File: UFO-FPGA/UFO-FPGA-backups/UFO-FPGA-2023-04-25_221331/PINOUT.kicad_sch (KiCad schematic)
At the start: 4 parts, among them J2 Power, J3 Digital, J4 Digital/PWM, J5 Digital

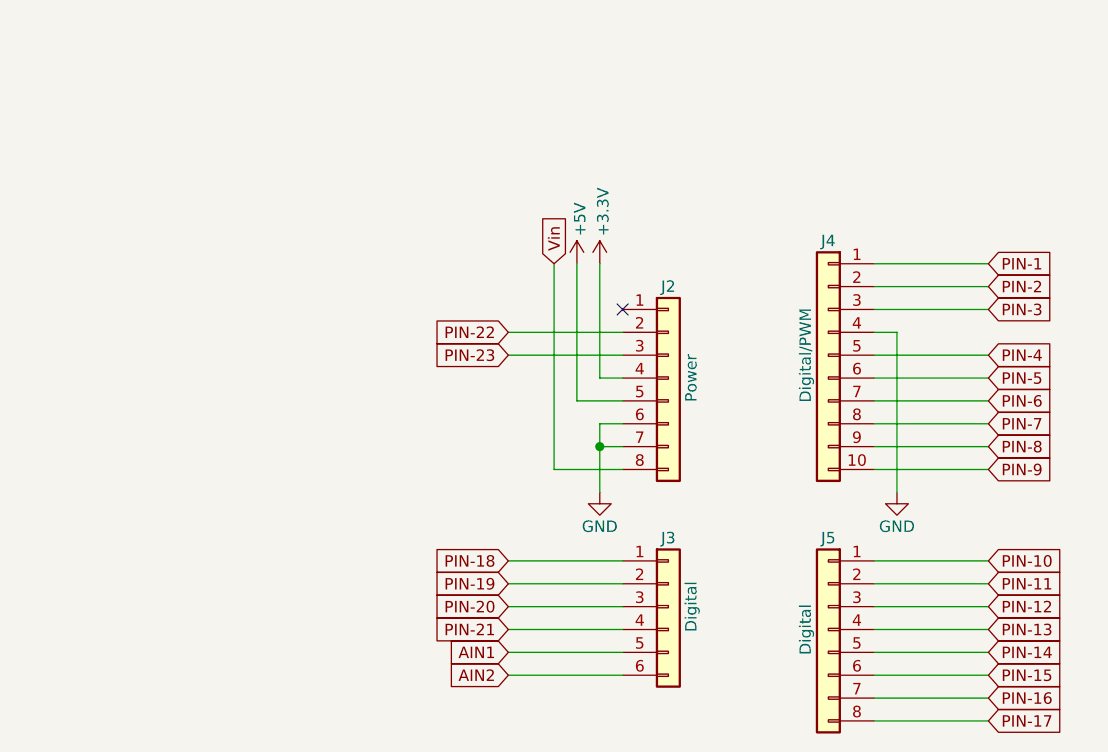
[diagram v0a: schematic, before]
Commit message: IO and power
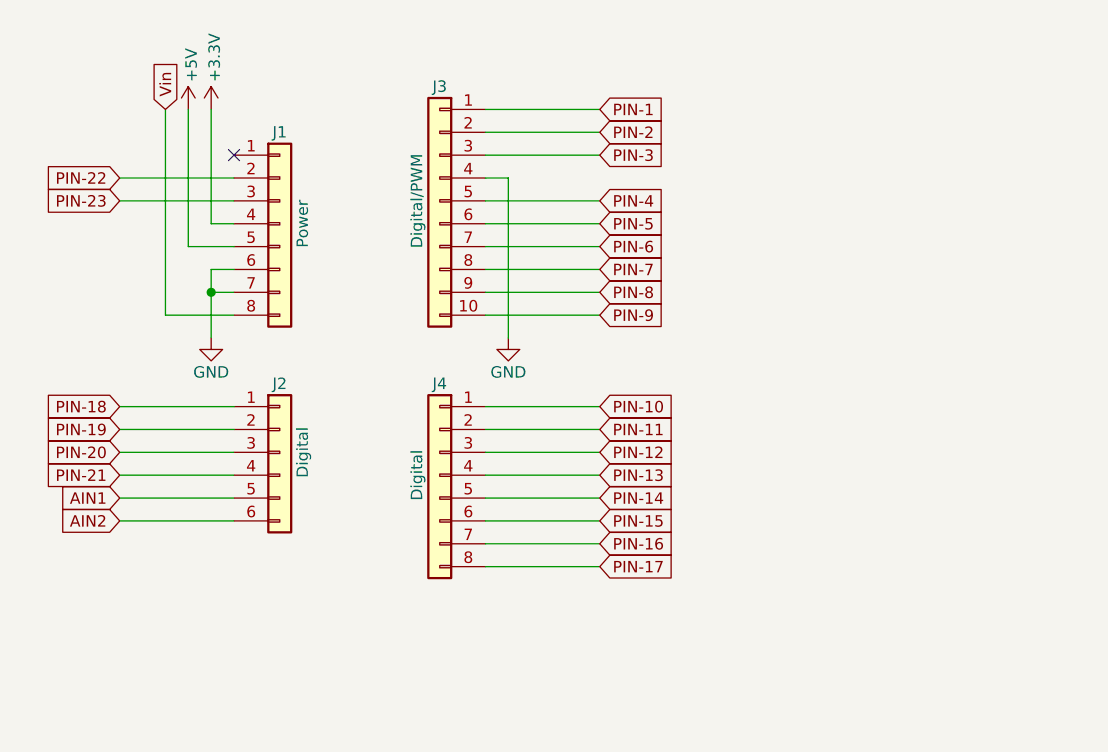
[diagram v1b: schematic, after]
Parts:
- removed J2: Power, Connector_PinSocket_2.54mm:PinSocket_1x08_P2.54mm_Vertical, symbol Connector_Generic:Conn_01x08
- removed J3: Digital, Connector_PinSocket_2.54mm:PinSocket_1x06_P2.54mm_Vertical, symbol Connector_Generic:Conn_01x06
- removed J4: Digital/PWM, Connector_PinSocket_2.54mm:PinSocket_1x10_P2.54mm_Vertical, symbol Connector_Generic:Conn_01x10
- removed J5: Digital, Connector_PinSocket_2.54mm:PinSocket_1x08_P2.54mm_Vertical, symbol Connector_Generic:Conn_01x08
- added J1: Power, Connector_PinSocket_2.54mm:PinSocket_1x08_P2.54mm_Vertical, symbol Connector_Generic:Conn_01x08
- added J2: Digital, Connector_PinSocket_2.54mm:PinSocket_1x06_P2.54mm_Vertical, symbol Connector_Generic:Conn_01x06
- added J3: Digital/PWM, Connector_PinSocket_2.54mm:PinSocket_1x10_P2.54mm_Vertical, symbol Connector_Generic:Conn_01x10
- added J4: Digital, Connector_PinSocket_2.54mm:PinSocket_1x08_P2.54mm_Vertical, symbol Connector_Generic:Conn_01x08
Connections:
- net +3V3: now also J1.4 (Pin_4)
- net +5V: now also J1.5 (Pin_5)
- net AIN1: now also J2.5 (Pin_5)
- net AIN2: now also J2.6 (Pin_6)
- net GND: now also J1.6 (Pin_6), J1.7 (Pin_7), J3.4 (Pin_4)
- net PIN-1: now also J3.1 (Pin_1)
- net PIN-10: now also J4.1 (Pin_1)
- net PIN-11: now also J4.2 (Pin_2)
- net PIN-12: now also J4.3 (Pin_3)
- net PIN-13: now also J4.4 (Pin_4)
- net PIN-14: now also J4.5 (Pin_5)
- net PIN-15: now also J4.6 (Pin_6)
- net PIN-16: now also J4.7 (Pin_7)
- net PIN-17: now also J4.8 (Pin_8)
- net PIN-18: now also J2.1 (Pin_1)
- net PIN-19: now also J2.2 (Pin_2)
- net PIN-2: now also J3.2 (Pin_2)
- net PIN-20: now also J2.3 (Pin_3)
- net PIN-21: now also J2.4 (Pin_4)
- net PIN-22: now also J1.2 (Pin_2)
- net PIN-23: now also J1.3 (Pin_3)
- net PIN-3: now also J3.3 (Pin_3)
- net PIN-4: now also J3.5 (Pin_5)
- net PIN-5: now also J3.6 (Pin_6)
- net PIN-6: now also J3.7 (Pin_7)
- net PIN-7: now also J3.8 (Pin_8)
- net PIN-8: now also J3.9 (Pin_9)
- net PIN-9: now also J3.10 (Pin_10)
- net Vin: now also J1.8 (Pin_8)
